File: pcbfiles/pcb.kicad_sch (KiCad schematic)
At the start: 236 parts, among them J1 Conn_01x06, J2 Conn_01x06, J3 Conn_01x06, J4 Conn_01x06, J5 Conn_01x04_Female, J6 Conn_01x04_Female, Q1 AO3401A, Q2 AO3401A, SW1 SW_SPST, SW10 SW_SPST, SW11 SW_SPST, SW12 SW_SPST, SW13 SW_SPST, SW14 SW_SPST, SW15 SW_SPST, SW16 SW_SPST, SW17 SW_SPST, SW18 SW_SPST, SW19 SW_SPST, SW2 SW_SPST, SW20 SW_SPST, SW21 SW_SPST, SW22 SW_SPST, SW23 SW_SPST, SW24 SW_SPST, SW25 SW_SPST, SW26 SW_SPST, SW27 SW_SPST, SW28 SW_SPST, SW29 SW_SPST, SW3 SW_SPST, SW30 SW_SPST, SW31 SW_SPST, SW32 SW_SPST, SW33 SW_SPST, SW34 SW_SPST, SW35 SW_SPST, SW36 SW_SPST, SW37 SW_SPST, SW38 SW_SPST, SW39 SW_SPST, SW4 SW_SPST, SW40 SW_SPST, SW41 SW_SPST, SW42 SW_SPST, SW43 SW_SPST, SW44 SW_SPST, SW45 SW_SPST, SW46 SW_SPST, SW47 SW_SPST, SW48 SW_SPST, SW49 SW_SPST, SW5 SW_SPST, SW50 SW_SPST, SW51 SW_SPST, SW52 SW_SPST, SW53 SW_SPST, SW54 SW_SPST, SW55 SW_SPST, SW56 SW_SPST, SW57 SW_SPST, SW58 SW_SPST, SW59 SW_SPST, SW6 SW_SPST, SW60 SW_SPST, SW61 SW_SPST, SW62 SW_SPST, SW63 SW_SPST, SW64 SW_SPST, SW65 SW_SPST, SW66 SW_SPST, SW67 SW_SPST, SW68 SW_SPST, SW69 SW_SPST, SW7 SW_SPST, SW70 SW_SPST, SW71 SW_SPST, SW72 SW_SPST, SW73 SW_SPST, SW74 SW_SPST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

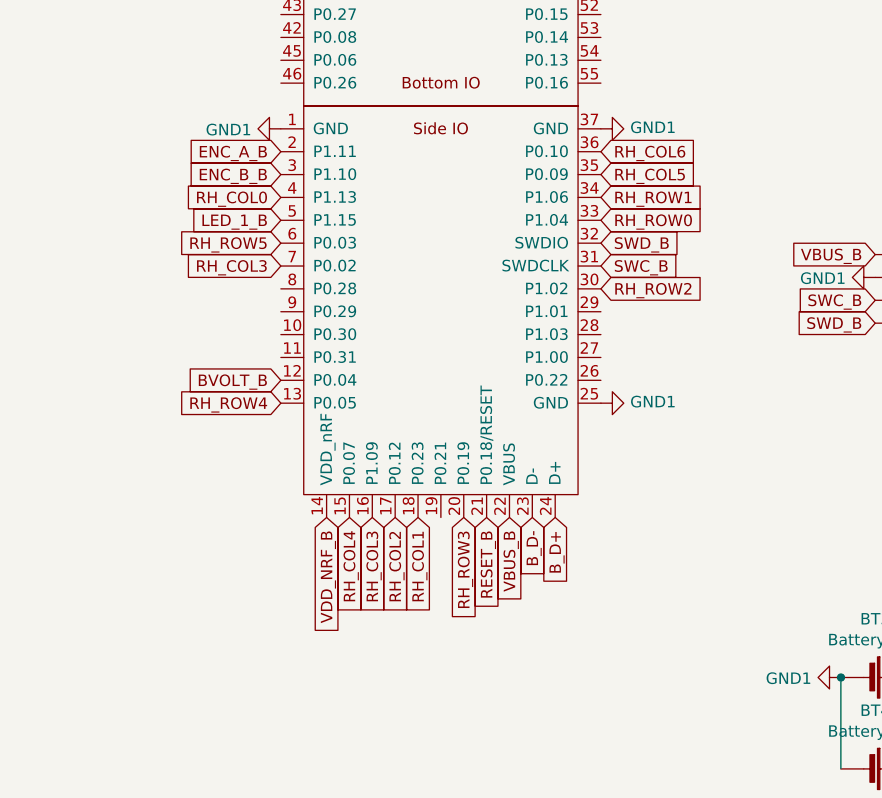
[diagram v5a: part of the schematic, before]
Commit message: Routing.
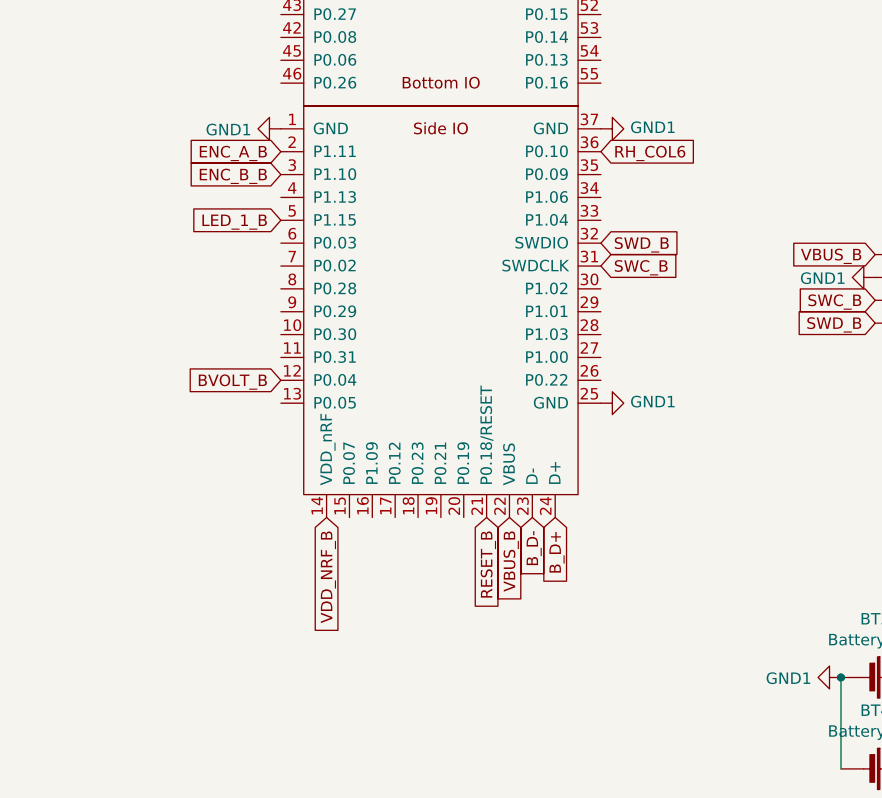
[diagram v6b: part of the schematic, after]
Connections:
- net ENC_P1_B: no longer U6.4 (P1.13)
- net RH_COL1: no longer U6.18 (P0.23)
- net RH_COL2: no longer U6.17 (P0.12)
- net RH_COL3: no longer U6.16 (P1.09), U6.7 (P0.02)
- net RH_COL4: no longer U6.15 (P0.07)
- net RH_COL5: no longer U6.35 (P0.09)
- net RH_ROW0: no longer U6.33 (P1.04)
- net RH_ROW1: no longer U6.34 (P1.06)
- net RH_ROW2: no longer U6.30 (P1.02)
- net RH_ROW3: no longer U6.20 (P0.19)
- net RH_ROW4: no longer U6.13 (P0.05)
- net RH_ROW5: no longer U6.6 (P0.03)
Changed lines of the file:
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@@
-    )
-  )
-  (global_label "RH_ROW0" (shape input) (at 525.272 255.27 0) (fields_autoplaced)
-    (effects (font (size 1.27 1.27)) (justify left))
-    (property "Intersheet References" "${INTERSHEET_REFS}" (id 0) (at 60.452 128.27 0)
-      (effects (font (size 1.27 1.27)) hide)
     )
   )
@@
     )
   )
-  (global_label "RH_COL3" (shape input) (at 499.872 288.29 270) (fields_autoplaced)
-    (effects (font (size 1.27 1.27)) (justify right))
-    (property "Intersheet References" "${INTERSHEET_REFS}" (id 0) (at 60.452 128.27 0)
-      (effects (font (size 1.27 1.27)) hide)
-    )
-  )
   (global_label "D-" (shape input) (at 64.262 288.29 270) (fields_autoplaced)
     (effects (font (size 1.27 1.27)) (justify right))
@@
     )
   )
-  (global_label "RH_COL4" (shape input) (at 497.332 288.29 270) (fields_autoplaced)
-    (effects (font (size 1.27 1.27)) (justify right))
-    (property "Intersheet References" "${INTERSHEET_REFS}" (id 0) (at 60.452 128.27 0)
-      (effects (font (size 1.27 1.27)) hide)
-    )
-  )
   (global_label "DBA_COL2" (shape input) (at 105.41 103.632 90) (fields_autoplaced)
     (effects (font (size 1.27 1.27)) (justify left))
@@
     (effects (font (size 1.27 1.27)) (justify left))
     (property "Intersheet References" "${INTERSHEET_REFS}" (id 0) (at 169.672 110.49 0)
-      (effects (font (size 1.27 1.27)) hide)
-    )
-  )
-  (global_label "RH_ROW2" (shape input) (at 525.272 262.89 0) (fields_autoplaced)
-    (effects (font (size 1.27 1.27)) (justify left))
-    (property "Intersheet References" "${INTERSHEET_REFS}" (id 0) (at 60.452 128.27 0)
       (effects (font (size 1.27 1.27)) hide)
     )
@@
     )
   )
-  (global_label "RH_COL5" (shape input) (at 525.272 250.19 0) (fields_autoplaced)
-    (effects (font (size 1.27 1.27)) (justify left))
-    (property "Intersheet References" "${INTERSHEET_REFS}" (id 0) (at 60.452 128.27 0)
-      (effects (font (size 1.27 1.27)) hide)
-    )
-  )
   (global_label "ENC_A" (shape input) (at 66.802 129.032 180) (fields_autoplaced)
     (effects (font (size 1.27 1.27)) (justify right))
@@
     )
   )
-  (global_label "RH_COL0" (shape input) (at 489.712 252.73 180) (fields_autoplaced)
-    (effects (font (size 1.27 1.27)) (justify right))
-    (property "Intersheet References" "${INTERSHEET_REFS}" (id 0) (at 60.452 128.27 0)
-      (effects (font (size 1.27 1.27)) hide)
-    )
-  )
-  (global_label "RH_ROW5" (shape input) (at 489.712 257.81 180) (fields_autoplaced)
-    (effects (font (size 1.27 1.27)) (justify right))
-    (property "Intersheet References" "${INTERSHEET_REFS}" (id 0) (at 60.452 128.27 0)
-      (effects (font (size 1.27 1.27)) hide)
-    )
-  )
   (global_label "DBA_P5" (shape input) (at 164.592 105.918 180) (fields_autoplaced)
     (effects (font (size 1.27 1.27)) (justify right))
@@
     (effects (font (size 1.27 1.27)) (justify right))
     (property "Intersheet References" "${INTERSHEET_REFS}" (id 0) (at 60.96 126.492 0)
-      (effects (font (size 1.27 1.27)) hide)
-    )
-  )
-  (global_label "RH_COL3" (shape input) (at 489.712 260.35 180) (fields_autoplaced)
-    (effects (font (size 1.27 1.27)) (justify right))
-    (property "Intersheet References" "${INTERSHEET_REFS}" (id 0) (at 60.452 128.27 0)
       (effects (font (size 1.27 1.27)) hide)
     )
@@
     )
   )
-  (global_label "RH_ROW3" (shape input) (at 510.032 288.29 270) (fields_autoplaced)
-    (effects (font (size 1.27 1.27)) (justify right))
-    (property "Intersheet References" "${INTERSHEET_REFS}" (id 0) (at 60.452 128.27 0)
-      (effects (font (size 1.27 1.27)) hide)
-    )
-  )
   (global_label "B_D-" (shape input) (at 531.622 156.21 0) (fields_autoplaced)
     (effects (font (size 1.27 1.27)) (justify left))
@@
     )
   )
-  (global_label "RH_COL1" (shape input) (at 504.952 288.29 270) (fields_autoplaced)
-    (effects (font (size 1.27 1.27)) (justify right))
-    (property "Intersheet References" "${INTERSHEET_REFS}" (id 0) (at 60.452 128.27 0)
-      (effects (font (size 1.27 1.27)) hide)
-    )
-  )
   (global_label "VBUS_B" (shape input) (at 555.752 259.08 180) (fields_autoplaced)
     (effects (font (size 1.27 1.27)) (justify right))
@@
     (effects (font (size 1.27 1.27)) (justify left))
     (property "Intersheet References" "${INTERSHEET_REFS}" (id 0) (at 60.96 126.492 0)
-      (effects (font (size 1.27 1.27)) hide)
-    )
-  )
-  (global_label "RH_COL2" (shape input) (at 502.412 288.29 270) (fields_autoplaced)
-    (effects (font (size 1.27 1.27)) (justify right))
-    (property "Intersheet References" "${INTERSHEET_REFS}" (id 0) (at 60.452 128.27 0)
       (effects (font (size 1.27 1.27)) hide)
     )
@@
     )
   )
-  (global_label "RH_ROW4" (shape input) (at 489.712 275.59 180) (fields_autoplaced)
-    (effects (font (size 1.27 1.27)) (justify right))
-    (property "Intersheet References" "${INTERSHEET_REFS}" (id 0) (at 60.452 128.27 0)
-      (effects (font (size 1.27 1.27)) hide)
-    )
-  )
   (global_label "BVOLT" (shape input) (at 36.322 273.05 180) (fields_autoplaced)
     (effects (font (size 1.27 1.27)) (justify right))
@@
       (effects (font (size 1.27 1.27)) hide)
     )
-  )
-  (global_label "RH_ROW1" (shape input) (at 525.272 252.73 0) (fields_autoplaced)
-    (effects (font (size 1.27 1.27)) (justify left))
-    (property "Intersheet References" "${INTERSHEET_REFS}" (id 0) (at 60.452 128.27 0)
-      (effects (font (size 1.27 1.27)) hide)
-    )
